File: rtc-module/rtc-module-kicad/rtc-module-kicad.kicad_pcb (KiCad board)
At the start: 2 copper layers, 45.5 x 36.4 mm, 11 parts, among them J1 Battery-holder, J2 Microcontroller, U1 PCF8563T

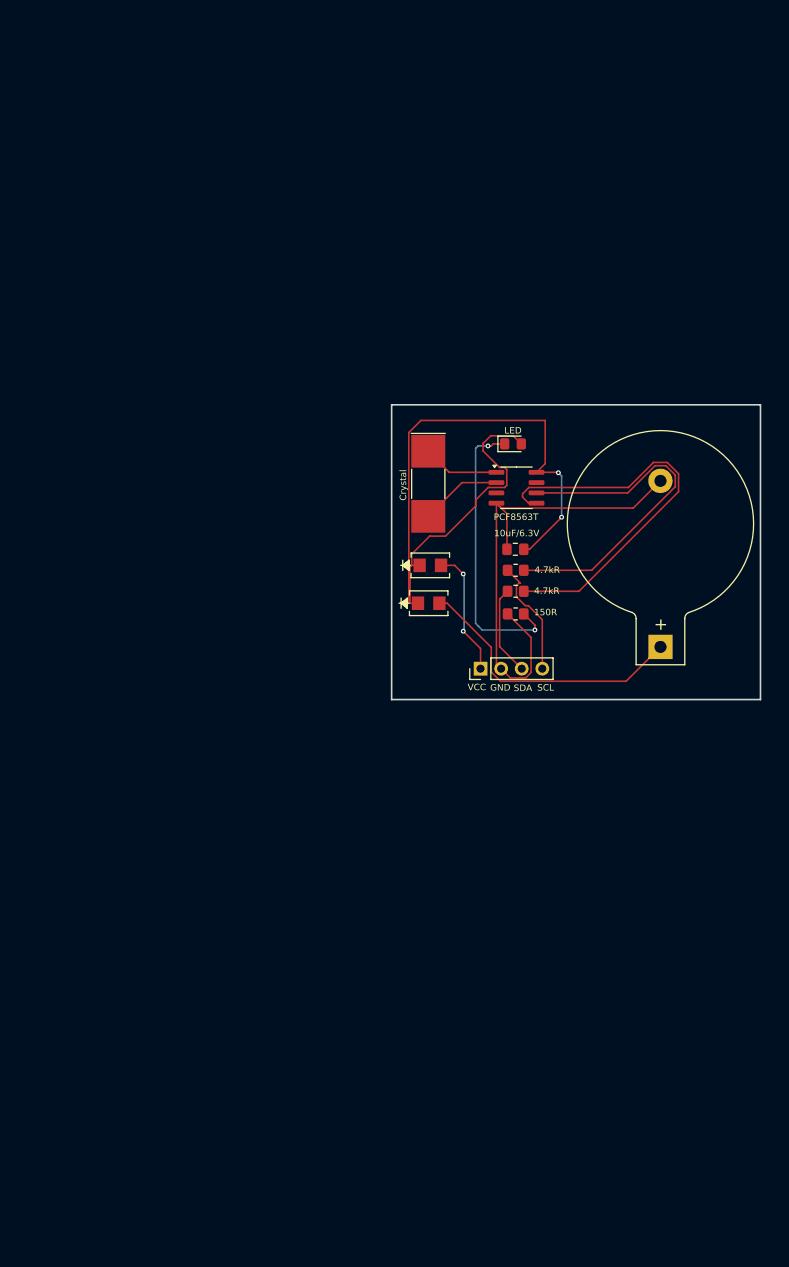
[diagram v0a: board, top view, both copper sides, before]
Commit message: Added the gerber and drill files ready to order!
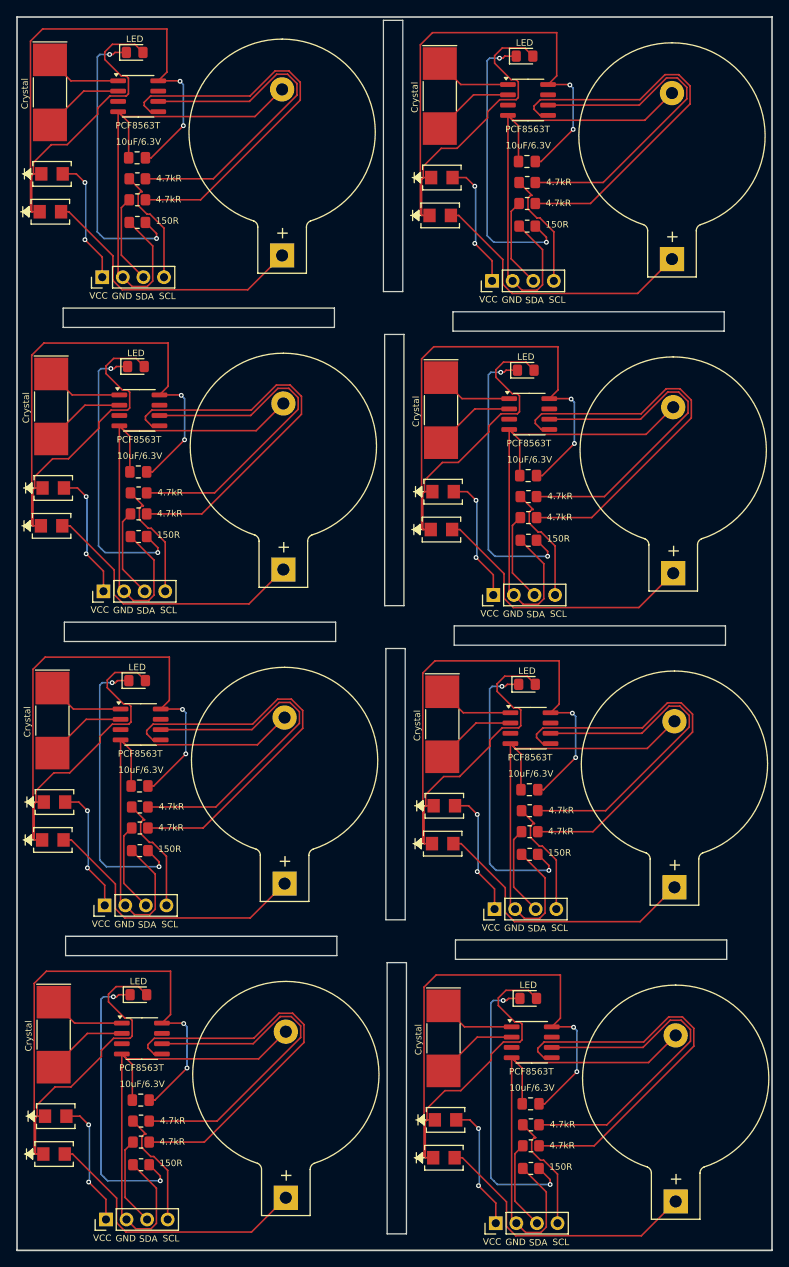
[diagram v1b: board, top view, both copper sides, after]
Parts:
- added 10uF/6.3V: C - 10uF/6.3V, Capacitor_SMD:C_0805_2012Metric_Pad1.18x1.45mm_HandSolder, F.Cu at (126.1, 164.4)
- added 10uF/6.3V: C - 10uF/6.3V, Capacitor_SMD:C_0805_2012Metric_Pad1.18x1.45mm_HandSolder, F.Cu at (77.9, 125.2)
- added 10uF/6.3V: C - 10uF/6.3V, Capacitor_SMD:C_0805_2012Metric_Pad1.18x1.45mm_HandSolder, F.Cu at (77.7, 86.4)
- added 10uF/6.3V: C - 10uF/6.3V, Capacitor_SMD:C_0805_2012Metric_Pad1.18x1.45mm_HandSolder, F.Cu at (125.8, 86.9)
- added 10uF/6.3V: C - 10uF/6.3V, Capacitor_SMD:C_0805_2012Metric_Pad1.18x1.45mm_HandSolder, F.Cu at (126.0, 125.6)
- added 10uF/6.3V: C - 10uF/6.3V, Capacitor_SMD:C_0805_2012Metric_Pad1.18x1.45mm_HandSolder, F.Cu at (125.7, 48.1)
- added 10uF/6.3V: C - 10uF/6.3V, Capacitor_SMD:C_0805_2012Metric_Pad1.18x1.45mm_HandSolder, F.Cu at (77.6, 47.7)
- added 150R: 150R, Resistor_SMD:R_0805_2012Metric_Pad1.20x1.40mm_HandSolder, F.Cu at (77.6, 55.6)
- added 150R: 150R, Resistor_SMD:R_0805_2012Metric_Pad1.20x1.40mm_HandSolder, F.Cu at (125.7, 56.1)
- added 150R: 150R, Resistor_SMD:R_0805_2012Metric_Pad1.20x1.40mm_HandSolder, F.Cu at (126.0, 133.6)
- added 150R: 150R, Resistor_SMD:R_0805_2012Metric_Pad1.20x1.40mm_HandSolder, F.Cu at (77.9, 133.1)
- added 150R: 150R, Resistor_SMD:R_0805_2012Metric_Pad1.20x1.40mm_HandSolder, F.Cu at (77.7, 94.4)
- added 150R: 150R, Resistor_SMD:R_0805_2012Metric_Pad1.20x1.40mm_HandSolder, F.Cu at (125.8, 94.8)
- added 150R: 150R, Resistor_SMD:R_0805_2012Metric_Pad1.20x1.40mm_HandSolder, F.Cu at (126.2, 172.4)
- added Crystal: Crystal - 32.768kHz, Crystal:Crystal_SMD_MicroCrystal_CC1V-T1A-2Pin_8.0x3.7mm_HandSoldering, F.Cu at (115.2, 117.6)
- added Crystal: Crystal - 32.768kHz, Crystal:Crystal_SMD_MicroCrystal_CC1V-T1A-2Pin_8.0x3.7mm_HandSoldering, F.Cu at (115.4, 156.3)
- added Crystal: Crystal - 32.768kHz, Crystal:Crystal_SMD_MicroCrystal_CC1V-T1A-2Pin_8.0x3.7mm_HandSoldering, F.Cu at (66.8, 39.6)
- added Crystal: Crystal - 32.768kHz, Crystal:Crystal_SMD_MicroCrystal_CC1V-T1A-2Pin_8.0x3.7mm_HandSoldering, F.Cu at (115.1, 78.8)
- added Crystal: Crystal - 32.768kHz, Crystal:Crystal_SMD_MicroCrystal_CC1V-T1A-2Pin_8.0x3.7mm_HandSoldering, F.Cu at (67.0, 78.3)
- added Crystal: Crystal - 32.768kHz, Crystal:Crystal_SMD_MicroCrystal_CC1V-T1A-2Pin_8.0x3.7mm_HandSoldering, F.Cu at (67.1, 117.1)
- added Crystal: Crystal - 32.768kHz, Crystal:Crystal_SMD_MicroCrystal_CC1V-T1A-2Pin_8.0x3.7mm_HandSoldering, F.Cu at (114.9, 40.0)
- added D1: Schottky-diode, SS14_Schottky:DO-214AC_VIS, F.Cu at (67.0, 93.1)
- added D1: Schottky-diode, SS14_Schottky:DO-214AC_VIS, F.Cu at (66.9, 54.3)
- added D1: Schottky-diode, SS14_Schottky:DO-214AC_VIS, F.Cu at (115.1, 93.5)
- added D1: Schottky-diode, SS14_Schottky:DO-214AC_VIS, F.Cu at (115.4, 171.0)
- added D1: Schottky-diode, SS14_Schottky:DO-214AC_VIS, F.Cu at (115.0, 54.8)
- added D1: Schottky-diode, SS14_Schottky:DO-214AC_VIS, F.Cu at (67.2, 131.8)
- added D1: Schottky-diode, SS14_Schottky:DO-214AC_VIS, F.Cu at (115.3, 132.3)
- added D2: Schottky-diode, SS14_Schottky:DO-214AC_VIS, F.Cu at (67.4, 127.2)
- added D2: Schottky-diode, SS14_Schottky:DO-214AC_VIS, F.Cu at (115.6, 166.4)
- added D2: Schottky-diode, SS14_Schottky:DO-214AC_VIS, F.Cu at (67.2, 88.4)
- added D2: Schottky-diode, SS14_Schottky:DO-214AC_VIS, F.Cu at (67.1, 49.6)
- added D2: Schottky-diode, SS14_Schottky:DO-214AC_VIS, F.Cu at (115.5, 127.6)
- added D2: Schottky-diode, SS14_Schottky:DO-214AC_VIS, F.Cu at (115.3, 88.8)
- added D2: Schottky-diode, SS14_Schottky:DO-214AC_VIS, F.Cu at (115.2, 50.1)
- added J1: Battery-holder, Battery:BatteryHolder_Keystone_103_1x20mm, F.Cu at (143.7, 98.9)
- added J1: Battery-holder, Battery:BatteryHolder_Keystone_103_1x20mm, F.Cu at (143.9, 137.7)
- added J1: Battery-holder, Battery:BatteryHolder_Keystone_103_1x20mm, F.Cu at (144.0, 176.4)
- added J1: Battery-holder, Battery:BatteryHolder_Keystone_103_1x20mm, F.Cu at (95.8, 137.2)
- added J1: Battery-holder, Battery:BatteryHolder_Keystone_103_1x20mm, F.Cu at (95.6, 98.5)
- added J1: Battery-holder, Battery:BatteryHolder_Keystone_103_1x20mm, F.Cu at (143.6, 60.2)
- added J1: Battery-holder, Battery:BatteryHolder_Keystone_103_1x20mm, F.Cu at (95.5, 59.7)
- added J2: Microcontroller, Connector_PinHeader_2.54mm:PinHeader_1x04_P2.54mm_Vertical, F.Cu at (73.6, 139.9)
- added J2: Microcontroller, Connector_PinHeader_2.54mm:PinHeader_1x04_P2.54mm_Vertical, F.Cu at (121.5, 101.6)
- added J2: Microcontroller, Connector_PinHeader_2.54mm:PinHeader_1x04_P2.54mm_Vertical, F.Cu at (121.4, 62.8)
- added J2: Microcontroller, Connector_PinHeader_2.54mm:PinHeader_1x04_P2.54mm_Vertical, F.Cu at (73.3, 62.4)
- added J2: Microcontroller, Connector_PinHeader_2.54mm:PinHeader_1x04_P2.54mm_Vertical, F.Cu at (121.7, 140.4)
- added J2: Microcontroller, Connector_PinHeader_2.54mm:PinHeader_1x04_P2.54mm_Vertical, F.Cu at (121.8, 179.1)
- added J2: Microcontroller, Connector_PinHeader_2.54mm:PinHeader_1x04_P2.54mm_Vertical, F.Cu at (73.4, 101.1)
- added LED: LED, LED_SMD:LED_0805_2012Metric_Pad1.15x1.40mm_HandSolder, F.Cu at (77.3, 34.6)
- added LED: LED, LED_SMD:LED_0805_2012Metric_Pad1.15x1.40mm_HandSolder, F.Cu at (125.7, 112.6)
- added LED: LED, LED_SMD:LED_0805_2012Metric_Pad1.15x1.40mm_HandSolder, F.Cu at (77.4, 73.4)
- added LED: LED, LED_SMD:LED_0805_2012Metric_Pad1.15x1.40mm_HandSolder, F.Cu at (125.5, 73.9)
- added LED: LED, LED_SMD:LED_0805_2012Metric_Pad1.15x1.40mm_HandSolder, F.Cu at (125.8, 151.4)
- added LED: LED, LED_SMD:LED_0805_2012Metric_Pad1.15x1.40mm_HandSolder, F.Cu at (125.4, 35.1)
- added LED: LED, LED_SMD:LED_0805_2012Metric_Pad1.15x1.40mm_HandSolder, F.Cu at (77.6, 112.2)
- added R1: 4.7kR, Resistor_SMD:R_0805_2012Metric_Pad1.20x1.40mm_HandSolder, F.Cu at (125.7, 53.3)
- added R1: 4.7kR, Resistor_SMD:R_0805_2012Metric_Pad1.20x1.40mm_HandSolder, F.Cu at (77.7, 91.6)
- added R1: 4.7kR, Resistor_SMD:R_0805_2012Metric_Pad1.20x1.40mm_HandSolder, F.Cu at (126.2, 169.6)
- added R1: 4.7kR, Resistor_SMD:R_0805_2012Metric_Pad1.20x1.40mm_HandSolder, F.Cu at (125.8, 92.0)
- added R1: 4.7kR, Resistor_SMD:R_0805_2012Metric_Pad1.20x1.40mm_HandSolder, F.Cu at (77.6, 52.8)
- added R1: 4.7kR, Resistor_SMD:R_0805_2012Metric_Pad1.20x1.40mm_HandSolder, F.Cu at (77.9, 130.4)
- added R1: 4.7kR, Resistor_SMD:R_0805_2012Metric_Pad1.20x1.40mm_HandSolder, F.Cu at (126.0, 130.8)
- added R2: 4.7kR, Resistor_SMD:R_0805_2012Metric_Pad1.20x1.40mm_HandSolder, F.Cu at (77.6, 50.2)
- added R2: 4.7kR, Resistor_SMD:R_0805_2012Metric_Pad1.20x1.40mm_HandSolder, F.Cu at (125.7, 50.7)
- added R2: 4.7kR, Resistor_SMD:R_0805_2012Metric_Pad1.20x1.40mm_HandSolder, F.Cu at (125.8, 89.5)
- added R2: 4.7kR, Resistor_SMD:R_0805_2012Metric_Pad1.20x1.40mm_HandSolder, F.Cu at (77.7, 89.0)
- added R2: 4.7kR, Resistor_SMD:R_0805_2012Metric_Pad1.20x1.40mm_HandSolder, F.Cu at (126.2, 167.0)
- added R2: 4.7kR, Resistor_SMD:R_0805_2012Metric_Pad1.20x1.40mm_HandSolder, F.Cu at (126.0, 128.2)
- added R2: 4.7kR, Resistor_SMD:R_0805_2012Metric_Pad1.20x1.40mm_HandSolder, F.Cu at (77.9, 127.8)
- added U1: PCF8563T, Package_SO:SOIC-8_3.9x4.9mm_P1.27mm, F.Cu at (126.3, 156.8)
- added U1: PCF8563T, Package_SO:SOIC-8_3.9x4.9mm_P1.27mm, F.Cu at (125.8, 40.5)
- added U1: PCF8563T, Package_SO:SOIC-8_3.9x4.9mm_P1.27mm, F.Cu at (78.0, 117.6)
- added U1: PCF8563T, Package_SO:SOIC-8_3.9x4.9mm_P1.27mm, F.Cu at (125.9, 79.3)
- added U1: PCF8563T, Package_SO:SOIC-8_3.9x4.9mm_P1.27mm, F.Cu at (126.1, 118.0)
- added U1: PCF8563T, Package_SO:SOIC-8_3.9x4.9mm_P1.27mm, F.Cu at (77.7, 40.1)
- added U1: PCF8563T, Package_SO:SOIC-8_3.9x4.9mm_P1.27mm, F.Cu at (77.8, 78.8)
- moved D2 82.2 mm to (67.5, 165.9)
- moved R1 82.2 mm to (78.0, 169.1)
- moved R2 82.2 mm to (78.0, 166.5)
- moved 10uF/6.3V 82.2 mm to (78.0, 163.9)
- moved 150R 82.2 mm to (78.0, 171.9)
- moved Crystal 82.2 mm to (67.3, 155.9)
- moved D1 82.2 mm to (67.3, 170.6)
- moved J1 82.2 mm to (95.9, 176.0)
- moved J2 82.2 mm to (73.7, 178.7)
- moved LED 82.2 mm to (77.7, 150.9)
- moved U1 82.2 mm to (78.1, 156.3)
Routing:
- net Net-(D1-K): track 96.1 -> 769.1 mm, vias 2 -> 16
- net Net-(J1-Pin_2): track 61.6 -> 493.2 mm
- net Net-(U1-SDA): track 50.3 -> 402.3 mm
- net Net-(U1-SCL): track 43.4 -> 347.1 mm
- net Net-(D3-K): track 35.6 -> 284.9 mm, vias 2 -> 16
- net Net-(D1-A): track 34.8 -> 278.4 mm
- net Net-(D2-A): track 15.8 -> 126.7 mm, vias 2 -> 16
- net Net-(J2-Pin_4): track 14.6 -> 117.2 mm
- net Net-(J2-Pin_3): track 11.1 -> 88.7 mm
- net Net-(U1-OSCO): track 10.1 -> 81.1 mm
- net Net-(U1-OSCI): track 9.48 -> 75.9 mm
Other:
- board size 45.5 x 36.4 mm -> 93.2 x 152.2 mm
- board text added: "Paco :3"
- board text added: "RTC-module"
